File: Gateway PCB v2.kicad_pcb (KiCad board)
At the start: 4 copper layers, 85 x 41 mm, 114 parts, among them J1 Conn_Coaxial, J2 Conn_01x04_Pin, J3 Conn_02x03_Odd_Even, J4 Conn_01x03_Pin, U6 TPS7A91, U7 TLV62568ADRL, X1 TG2016SMN 32.0000M-TCGNNMB

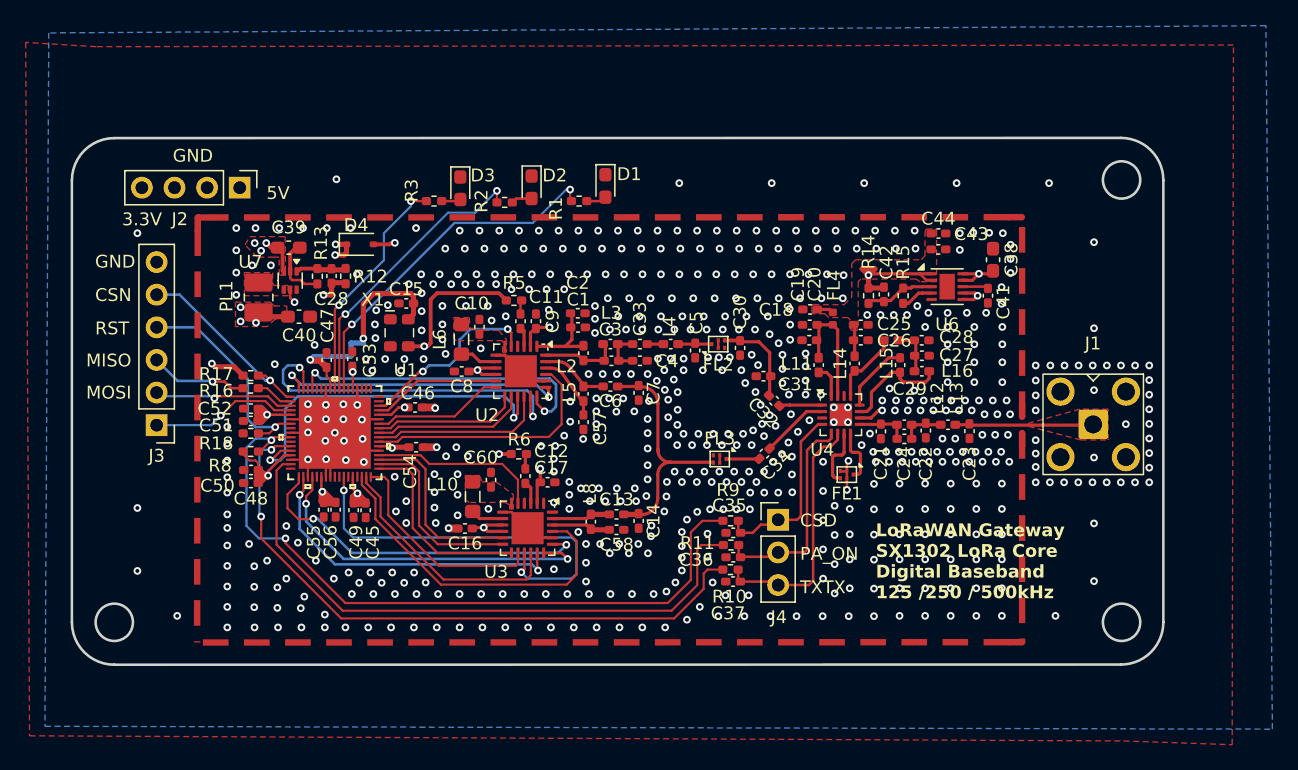
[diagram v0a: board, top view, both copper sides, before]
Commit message: Success
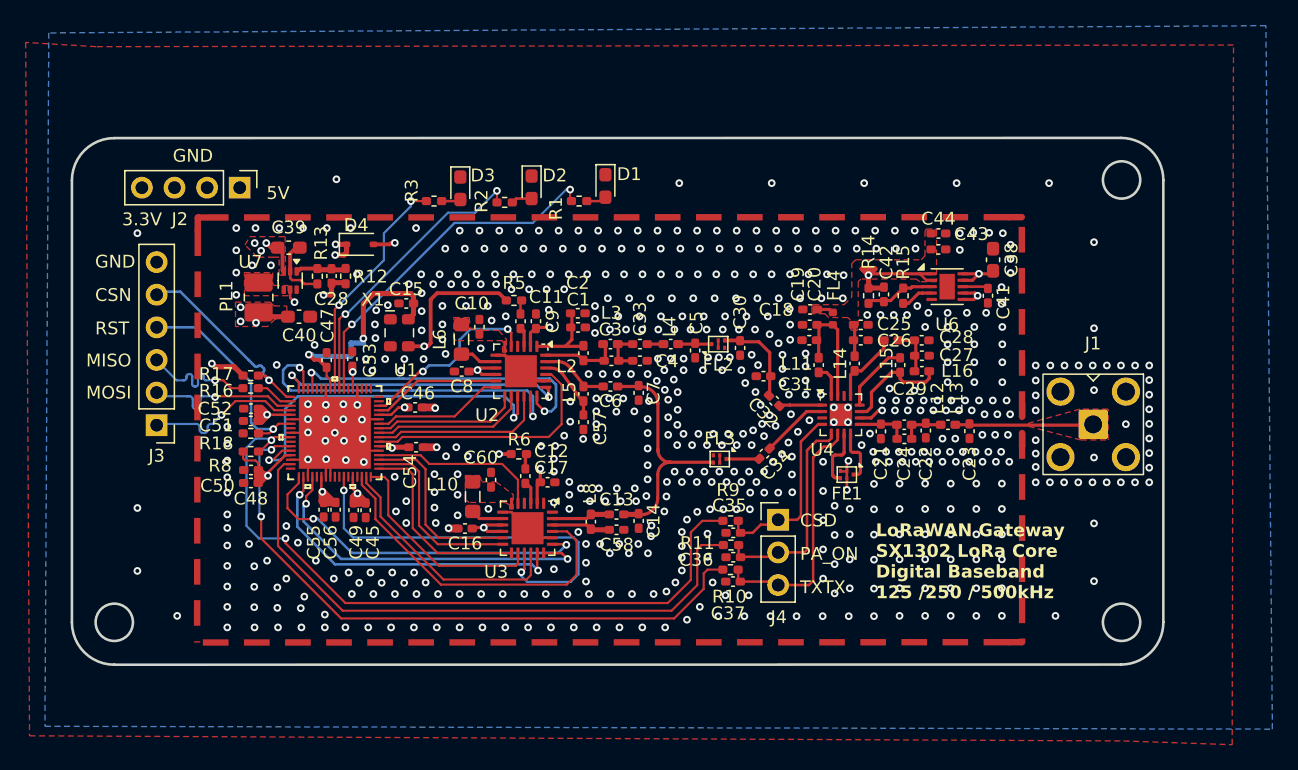
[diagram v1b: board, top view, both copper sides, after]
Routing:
- net EX_HOST_MISO: track 7.63 -> 10.1 mm
- net EX_HOST_MOSI: track 11.0 -> 12.5 mm
- net 3.3V: track 135.0 -> 135.9 mm
- net RADIOB_RESET: track 31.2 -> 31.9 mm
- net EX_HOST_CSN: track 14.8 -> 15.3 mm
- net EX_HOST_SCK: track 11.9 -> 12.5 mm
